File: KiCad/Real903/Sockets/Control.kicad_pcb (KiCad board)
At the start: 4 copper layers, 80 x 105 mm, 6 parts

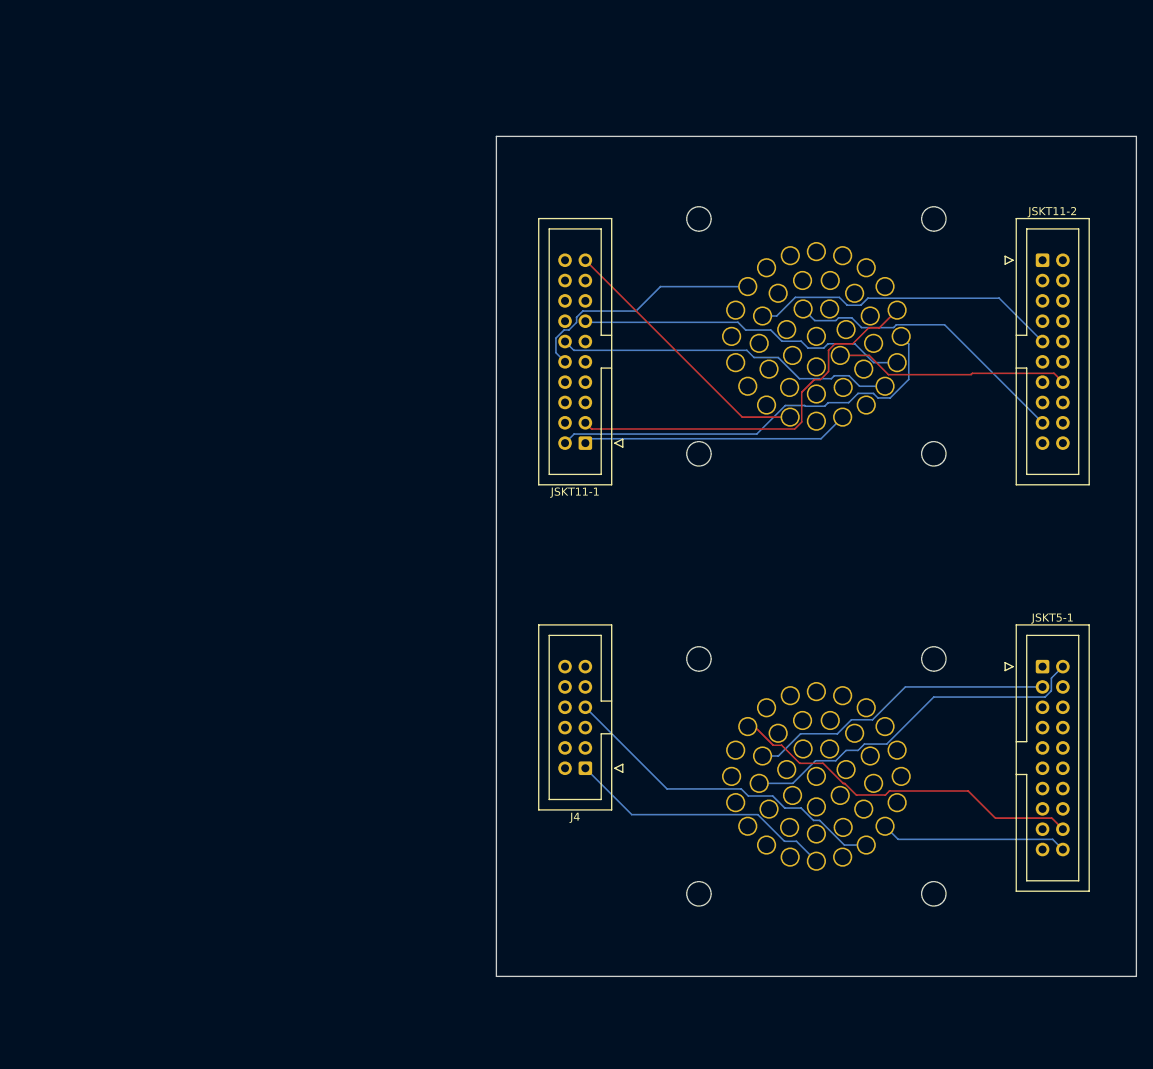
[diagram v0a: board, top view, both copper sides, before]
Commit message: September 4
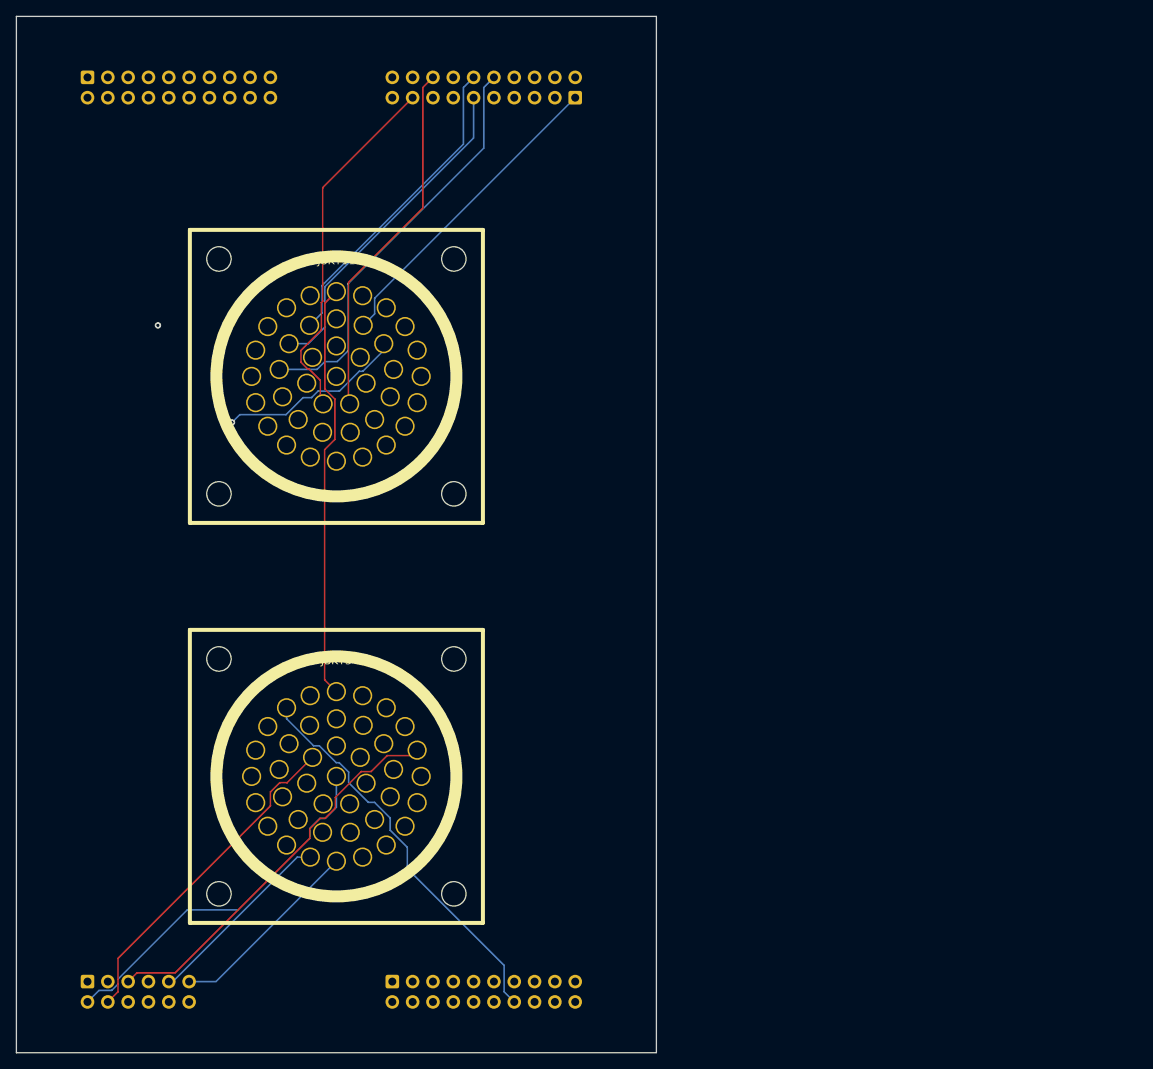
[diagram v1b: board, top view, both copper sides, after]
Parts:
- J4, JSKT11-1, JSKT11-2, JSKT5-1: moved to B.Cu
- JSKT11, JSKT5: moved to F.Cu
- moved JSKT5-1 90.3 mm to (47.0, 120.7), turned to 270 degrees
- moved JSKT11-1 77.2 mm to (8.89, 7.62), turned to 270 degrees
- moved J4 67.7 mm to (8.89, 120.7), turned to 270 degrees
- moved JSKT11-2 61.9 mm to (69.8, 10.2), turned to 90 degrees
- moved JSKT11 60.2 mm to (40.0, 45.0)
- moved JSKT5 60.0 mm to (40.0, 95.0)
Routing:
- net /Control Unit/AUDIO-32-14: track 50.3 -> 112.7 mm
- net /Control Unit/~SMN~-4-7: track 68.8 -> 35.1 mm
- net /Control Unit/AUT: track 67.6 -> 100.3 mm, vias 0 -> 1
- net /Control Unit/Auto-Start: track 57.7 -> 89.6 mm
- net GND: track 91.6 -> 118.6 mm
- net /Control Unit/AUTO-1-L: track 62.2 -> 88.9 mm
- net /Control Unit/W6: track 49.2 -> 75.1 mm
- net /Control Unit/ONG-1-7: track 39.0 -> 63.9 mm
- net /Control Unit/~TEST~-1-5: track 23.4 -> 43.6 mm
- net /Control Unit/~ONG~-1-F: track 39.0 -> 58.9 mm
- net /Control Unit/On: track 37.8 -> 57.3 mm
- net /Control Unit/W5: track 52.6 -> 71.9 mm
- net /Control Unit/~W~15: track 20.1 -> 39.4 mm
- net /Control Unit/~RESTART~-1-3: track 44.2 -> 62.7 mm
- net /Control Unit/W12: track 35.3 -> 53.6 mm
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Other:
- board size 80 x 105 mm -> 80 x 129.5 mm
